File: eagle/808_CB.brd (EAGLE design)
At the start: 100 x 80 mm, 54 parts, among them IC1 4584N, IC2 TL072P, Q1 2N3904, Q2 2N3904, Q3 2N3904, Q4 2N3906, X1 22-23-2021

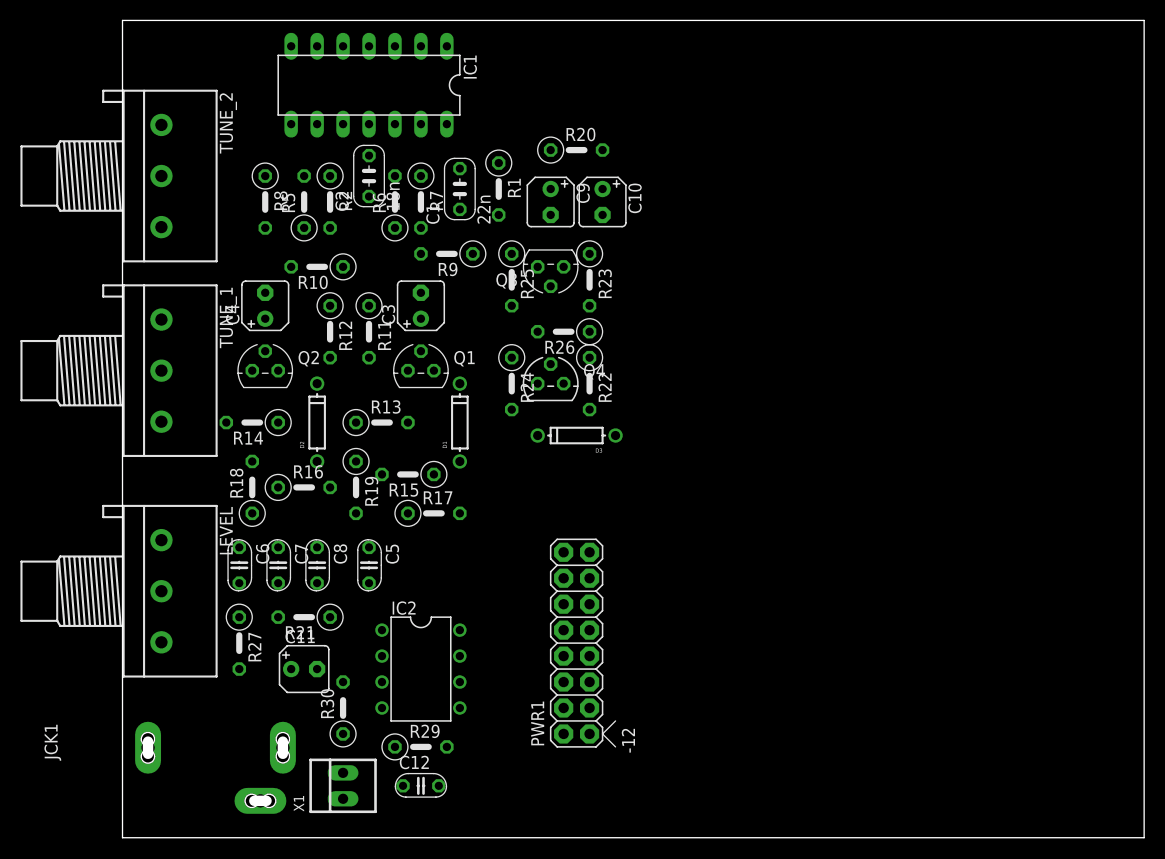
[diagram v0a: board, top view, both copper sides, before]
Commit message: routed
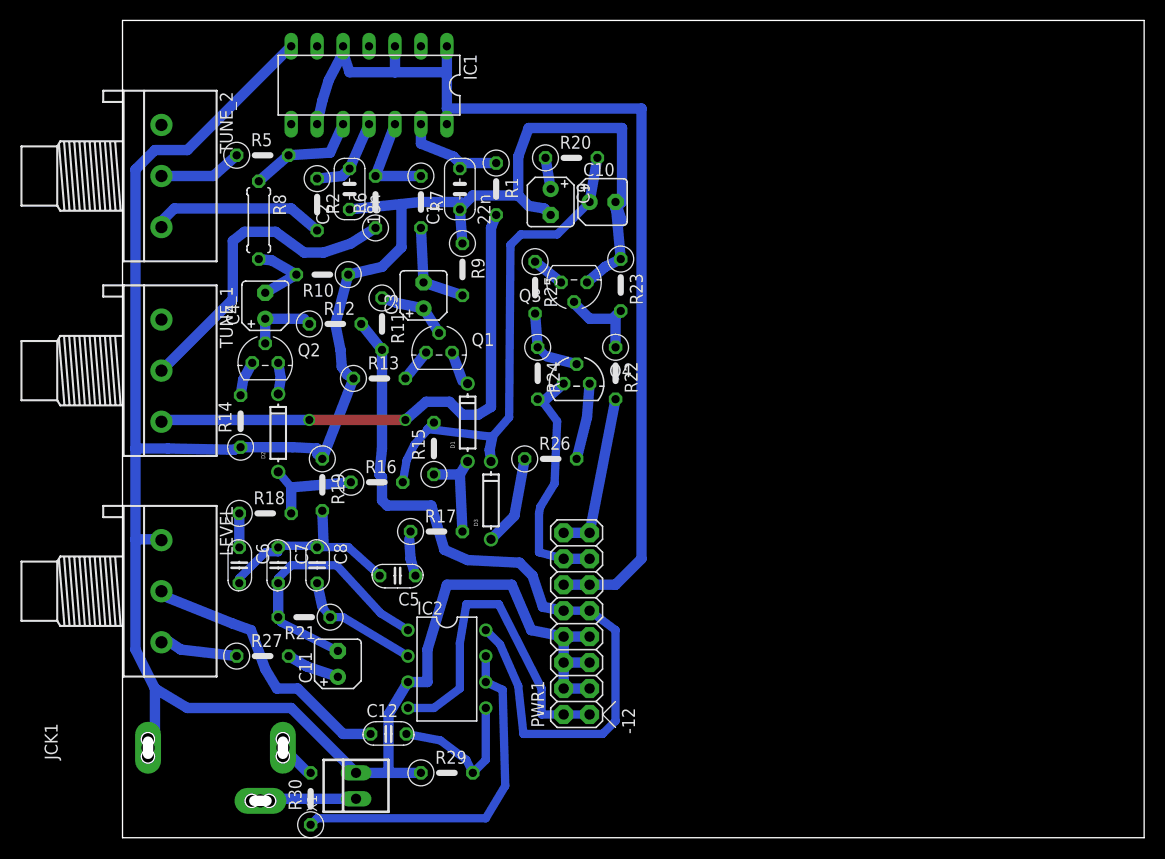
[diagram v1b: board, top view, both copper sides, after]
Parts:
- R8: device TR808clone:0207/5V -> TR808clone:0207/7
- moved R26 12.5 mm to (41.9, 37.1), turned to 0 degrees
- moved D3 10.5 mm to (36.1, 33.0), turned to 90 degrees
- moved R30 9.44 mm to (18.4, 3.81)
- moved R16 7.13 mm to (24.9, 34.8)
- moved R5 6.12 mm to (13.7, 66.8), turned to 0 degrees
- moved C12 5.99 mm to (26.0, 10.2)
- moved R13 4.33 mm to (25.1, 45.0)
- moved D2 3.94 mm to (15.2, 39.6)
- moved R29 3.59 mm to (31.8, 6.35)
- moved R15 3.59 mm to (30.5, 38.1), turned to 90 degrees
- moved C11 3.34 mm to (21.1, 17.0), turned to 90 degrees
- moved R19 3.31 mm to (19.6, 34.5)
- moved R23 3.09 mm to (48.8, 54.1)
- moved C5 2.97 mm to (26.9, 25.7), turned to 180 degrees
- moved R18 2.84 mm to (14.0, 31.8), turned to 0 degrees
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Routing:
- net GND: track 0.00 -> 268.4 mm
- net +5V: track 0.00 -> 101.6 mm
- net +15V: track 0.00 -> 77.6 mm
- net N$7: track 0.00 -> 52.6 mm, vias 0 -> 2
- net N$17: track 0.00 -> 49.8 mm
- net N$33: track 0.00 -> 34.9 mm
- net -15V: track 0.00 -> 33.7 mm
- net N$5: track 0.00 -> 31.1 mm
- net N$31: track 0.00 -> 26.9 mm
- net N$27: track 0.00 -> 26.4 mm
- net TRIG*: track 0.00 -> 23.9 mm
- net N$25: track 0.00 -> 21.2 mm
- net N$8: track 0.00 -> 17.1 mm
- net LT: track 0.00 -> 15.9 mm
- net N$32: track 0.00 -> 14.9 mm
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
